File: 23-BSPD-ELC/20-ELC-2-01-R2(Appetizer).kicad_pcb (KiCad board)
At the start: 2 copper layers, 152.4 x 60.8 mm, 221 parts, among them J1 Conn_02x08_Counter_Clockwise, J2 Conn_01x02, J3 Conn_01x02, J4 SWD, Q1 Q_PMOS_GSD, Q2 Q_PMOS_GSD, Q3 Q_NMOS_GSD-Device, Q4 Q_NMOS_GSD-Device, Q5 Q_NMOS_GSD-Device, Q6 Q_NMOS_GSD-Device, Q7 Q_PMOS_DSG, Q8 Q_PMOS_DSG, SW1 SW_SPDT, U1 SN74ALS32DR, U10 LM239, U11 LM239, U13 LM239, U15 LM239, U16 STM32F105RCTx, U17 SN65HVD230, U18 SN65HVD230, U19 LMR51420, U2 74HC04D,653, U20 AMS1117-3.3, U3 74HC08D,653, U4 74LVC2G17DBVE4, U5 APX823-44W5G-7, U6 CD4043BDR, U8 LM239, Y1 16MHz

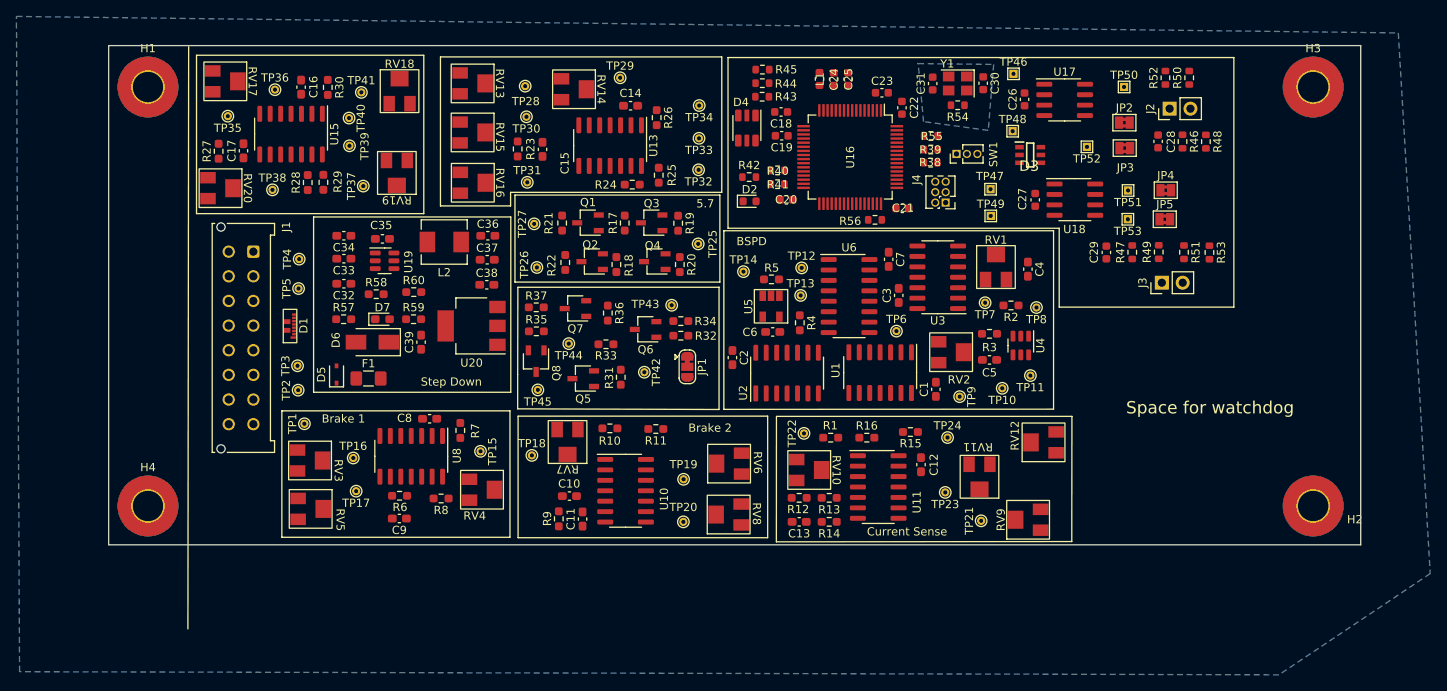
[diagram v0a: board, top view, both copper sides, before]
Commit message: BSPD layout
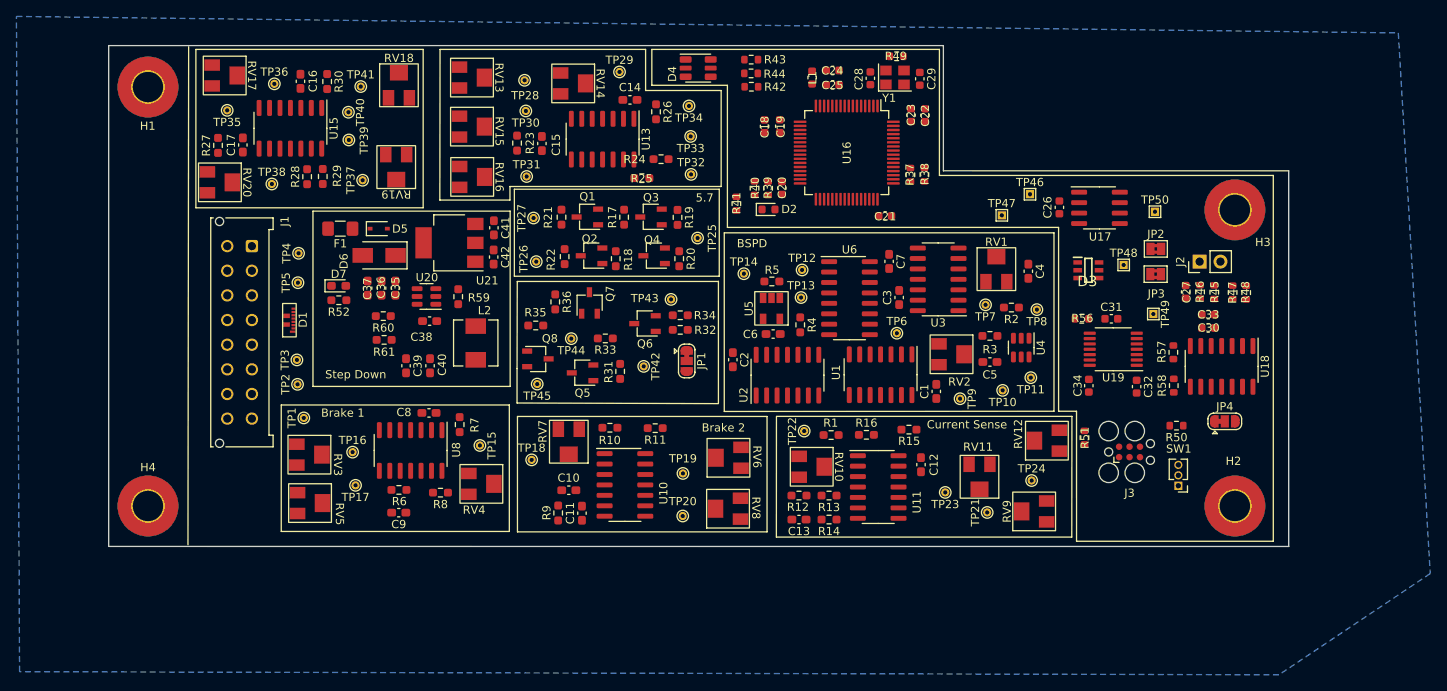
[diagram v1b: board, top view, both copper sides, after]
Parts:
- removed J4: SWD, Connector_PinHeader_1.27mm:PinHeader_2x03_P1.27mm_Vertical
- removed JP5: , Jumper:SolderJumper-2_P1.3mm_Bridged2Bar_Pad1.0x1.5mm
- removed R53: 120, Resistor_SMD:R_0603_1608Metric
- removed R54: 47, Resistor_SMD:R_0603_1608Metric
- removed R55: 10K, Resistor_SMD:R_0603_1608Metric
- removed TP51, TP52, TP53: , TestPoint:TestPoint_THTPad_1.0x1.0mm_Drill0.5mm
- added C40: 22uF, Capacitor_SMD:C_0603_1608Metric_Pad1.08x0.95mm_HandSolder, F.Cu at (106.3, 101.1)
- added C41: 1uF, Capacitor_SMD:C_0603_1608Metric_Pad1.08x0.95mm_HandSolder, F.Cu at (114.1, 84.3)
- added C42: 22uF, Capacitor_SMD:C_0603_1608Metric_Pad1.08x0.95mm_HandSolder, F.Cu at (114.1, 87.8)
- added R61: 54.9K, Resistor_SMD:R_0603_1608Metric_Pad0.98x0.95mm_HandSolder, F.Cu at (100.8, 97.9)
- added U21: AMS1117-3.3, Package_TO_SOT_SMD:SOT-223-3_TabPin2, F.Cu at (108.7, 86.1)
- C27: value 0u1 -> 4.7n
- C28, C29: value 4.7n -> 10p
- C30: value 10p -> .1uF
- C31: value 10p -> 1uF
- C32: value 10uF -> .1uF; footprint Capacitor_SMD:C_0603_1608Metric_Pad1.08x0.95mm_HandSolder -> Capacitor_SMD:C_0603_1608Metric
- C33: footprint Capacitor_SMD:C_0603_1608Metric_Pad1.08x0.95mm_HandSolder -> Capacitor_SMD:C_0603_1608Metric
- C34: value 100nF -> .1uF; footprint Capacitor_SMD:C_0603_1608Metric_Pad1.08x0.95mm_HandSolder -> Capacitor_SMD:C_0603_1608Metric
- C35: value 100nF -> 10uF
- C36: value 22uF -> 10uF
- C37: value 22uF -> 100nF
- C38: value 1uF -> 100nF
- J3: value Conn_01x02 -> SWD; footprint Connector_PinHeader_2.54mm:PinHeader_1x02_P2.54mm_Vertical -> Connector:Tag-Connect_TC2030-IDC-FP_2x03_P1.27mm_Vertical
- JP4: value (none) -> Jumper_3_Bridged12; footprint Jumper:SolderJumper-2_P1.3mm_Bridged2Bar_Pad1.0x1.5mm -> Jumper:SolderJumper-3_P1.3mm_Bridged12_RoundedPad1.0x1.5mm
- R19: value 250 -> 10k
- R37: value 25 -> 2k2; footprint Resistor_SMD:R_0603_1608Metric_Pad0.98x0.95mm_HandSolder -> Resistor_SMD:R_0603_1608Metric
- R41: value 2k2 -> 100
- R42: value 100 -> 220
- R45: value 220 -> 120
- R49: value 120 -> 47
- R50: value 120 -> 10K
- R51: value 120 -> 22
- R52: value 120 -> 470R; footprint Resistor_SMD:R_0603_1608Metric -> Resistor_SMD:R_0603_1608Metric_Pad0.98x0.95mm_HandSolder
- R56: value 22 -> 100k
- R57: value 470R -> 10k; footprint Resistor_SMD:R_0603_1608Metric_Pad0.98x0.95mm_HandSolder -> Resistor_SMD:R_0603_1608Metric
- R58: value 10K -> 10k; footprint Resistor_SMD:R_0603_1608Metric_Pad0.98x0.95mm_HandSolder -> Resistor_SMD:R_0603_1608Metric
- R60: value 54.9K -> 10K
- U18: value SN65HVD230 -> MCP3428; footprint Package_SO:SOIC-8_3.9x4.9mm_P1.27mm -> Package_SO:SOIC-14_3.9x8.7mm_P1.27mm
- U19: value LMR51420 -> LSF0204QPWRQ1; footprint Package_TO_SOT_SMD:SOT-23-6 -> Package_SO:TSSOP-14_4.4x5mm_P0.65mm
- U20: value AMS1117-3.3 -> LMR51420; footprint Package_TO_SOT_SMD:SOT-223-3_TabPin2 -> Package_TO_SOT_SMD:SOT-23-6
- moved C33 105.4 mm to (201.1, 94.8), turned to 0 degrees
- moved R52 104.2 mm to (95.2, 93.1), turned to 180 degrees
- moved R57 101.1 mm to (196.8, 99.4), turned to -90 degrees
- moved R58 97.7 mm to (196.9, 103.5), turned to 90 degrees
- moved C32 97.3 mm to (192.4, 103.6), turned to -90 degrees
- moved C34 92.5 mm to (186.5, 103.5), turned to -90 degrees
- moved U19 89.3 mm to (189.5, 99.1), turned to 180 degrees
- moved R45 61.3 mm to (201.8, 92.1), turned to -90 degrees
- moved SW1 48.6 mm to (197.4, 115.7), turned to 180 degrees
- moved R37 48.3 mm to (164.8, 77.8), turned to 90 degrees
- moved R50 42.4 mm to (197.2, 108.4), turned to 180 degrees
- moved C30 40.5 mm to (201.1, 96.5), turned to 0 degrees
- moved R49 39.8 mm to (163.1, 63.4), turned to 0 degrees
- moved C31 36.0 mm to (189.3, 95.4), turned to 0 degrees
- moved C28 35.9 mm to (159.9, 66.1)
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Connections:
- net /5.7/microcontroller/CAN1_H renamed /5.7/CANH
- net /5.7/microcontroller/CAN1_L renamed /5.7/CANL
- C27 pad 1: +3V3 -> GND
- C27 pad 2: GND -> Net-(C27-Pad2)
- C28 pad 1: GND -> /5.7/microcontroller/HSE_in
- C28 pad 2: Net-(C28-Pad2) -> GND
- C29 pad 1: GND -> Net-(C29-Pad1)
- C29 pad 2: Net-(C29-Pad2) -> GND
- C30 pad 1: /5.7/microcontroller/HSE_in -> +5V
- C32 pad 1: /24 to 5V Step Down/BUCK/V_in -> +3V3
- C33 pad 1: /24 to 5V Step Down/BUCK/V_in -> +5V
- C34 pad 1: /24 to 5V Step Down/BUCK/V_in -> +5V
- C35 pad 1: /24 to 5V Step Down/BUCK/SW -> /24 to 5V Step Down/BUCK/V_in
- C35 pad 2: /24 to 5V Step Down/BUCK/VBST -> GND
- C36 pad 1: +5V -> /24 to 5V Step Down/BUCK/V_in
- C37 pad 1: +5V -> /24 to 5V Step Down/BUCK/V_in
- C38 pad 1: +5V -> /24 to 5V Step Down/BUCK/SW
- C38 pad 2: GND -> /24 to 5V Step Down/BUCK/VBST
- C39 pad 1: +3V3 -> +5V
- D3 pad 1: Net-(D3-Pad1) -> unconnected-(D3-Pad1)
- D3 pad 3: Net-(D3-Pad3) -> unconnected-(D3-Pad3)
- J2 pad 1: Net-(C28-Pad2) -> Net-(C27-Pad2)
- J3 pad 1: Net-(C29-Pad2) -> +3V3
- JP4 pad 1: Net-(D3-Pad3) -> unconnected-(JP4-Pad1)
- JP4 pad 2: /5.7/microcontroller/CAN2_H -> Net-(JP4-Pad2)
- Q1 pad 3: /APPs1_Out -> /5.7/APPs1_Out
- Q2 pad 3: /APPs2_Out -> /5.7/APPs2_Out
- Q7 pad 2: /Shutdown_IN -> Net-(Q7-Pad2)
- Q7 pad 3: Net-(Q7-Pad3) -> /Shutdown_IN
- Q8 pad 2: Net-(Q8-Pad2) -> /Shutdown_OUT
- Q8 pad 3: /Shutdown_OUT -> Net-(Q7-Pad2)
- R21 pad 2: /APPs1_Out -> /5.7/APPs1_Out
- R22 pad 2: /APPs2_Out -> /5.7/APPs2_Out
- R35 pad 1: Net-(Q8-Pad2) -> Net-(Q7-Pad2)
- R37 pad 1: Net-(Q7-Pad3) -> +3V3
- R37 pad 2: Net-(Q8-Pad2) -> /5.7/microcontroller/I2C1_SCL
- R38 pad 2: /5.7/microcontroller/I2C1_SCL -> /5.7/microcontroller/I2C1_SDA
- R39 pad 2: /5.7/microcontroller/I2C1_SDA -> /5.7/microcontroller/I2C2_SCL
- R40 pad 2: /5.7/microcontroller/I2C2_SCL -> /5.7/microcontroller/I2C2_SDA
- R41 pad 1: +3V3 -> Net-(D2-Pad1)
- R41 pad 2: /5.7/microcontroller/I2C2_SDA -> GND
- R42 pad 1: Net-(D2-Pad1) -> Net-(D4-Pad6)
- R42 pad 2: GND -> /5.7/microcontroller/LED_B
- R43 pad 1: Net-(D4-Pad6) -> Net-(D4-Pad5)
- R43 pad 2: /5.7/microcontroller/LED_B -> /5.7/microcontroller/LED_G
- R44 pad 1: Net-(D4-Pad5) -> Net-(D4-Pad4)
- R44 pad 2: /5.7/microcontroller/LED_G -> /5.7/microcontroller/LED_R
- R45 pad 1: Net-(D4-Pad4) -> Net-(C27-Pad2)
- R45 pad 2: /5.7/microcontroller/LED_R -> Net-(D3-Pad4)
- R46 pad 1: Net-(C28-Pad2) -> Net-(C27-Pad2)
- R47 pad 1: Net-(C29-Pad2) -> Net-(D3-Pad6)
- R47 pad 2: Net-(D3-Pad1) -> Net-(J2-Pad2)
- R48 pad 1: Net-(C28-Pad2) -> Net-(D3-Pad6)
- R48 pad 2: Net-(D3-Pad4) -> Net-(J2-Pad2)
- R49 pad 1: Net-(C29-Pad2) -> /5.7/microcontroller/HSE_out
- R49 pad 2: Net-(D3-Pad1) -> Net-(C29-Pad1)
- R50 pad 1: Net-(D3-Pad6) -> Net-(R50-Pad1)
- R50 pad 2: Net-(J2-Pad2) -> /5.7/microcontroller/BOOT0
- R51 pad 1: Net-(D3-Pad3) -> Net-(J3-Pad2)
- R51 pad 2: Net-(J3-Pad2) -> /5.7/microcontroller/SWDIO
- R52 pad 1: Net-(D3-Pad6) -> GND
- R52 pad 2: Net-(J2-Pad2) -> Net-(D7-Pad1)
- R56 pad 1: Net-(J4-Pad2) -> Net-(C31-Pad1)
- R56 pad 2: /5.7/microcontroller/SWDIO -> +3V3
- R57 pad 1: GND -> /Watchdog/SDA
- R57 pad 2: Net-(D7-Pad1) -> +5V
- R58 pad 1: /24 to 5V Step Down/BUCK/V_in -> /Watchdog/SCL
- R58 pad 2: /24 to 5V Step Down/BUCK/EN -> +5V
- R59 pad 1: /24 to 5V Step Down/BUCK/VFB -> /24 to 5V Step Down/BUCK/V_in
- R59 pad 2: GND -> /24 to 5V Step Down/BUCK/EN
- R60 pad 2: +5V -> GND
- SW1 pad 2: Net-(R55-Pad1) -> Net-(R50-Pad1)
- TP1 pad 1: /Brake1_Signal_Raw -> /Brake2_Signal_Raw
- TP2 pad 1: /Current_Sense_Signal_Raw -> /Brake1_Signal_Raw
- TP26 pad 1: /APPs2_Out -> /5.7/APPs2_Out
- TP27 pad 1: /APPs1_Out -> /5.7/APPs1_Out
- TP3 pad 1: /Brake2_Signal_Raw -> /Current_Sense_Signal_Raw
- TP44 pad 1: Net-(Q7-Pad3) -> Net-(Q7-Pad2)
- TP47 pad 1: /5.7/microcontroller/CAN2_TX -> /5.7/microcontroller/CAN1_RX
- TP48 pad 1: /5.7/microcontroller/CAN1_RX -> Net-(D3-Pad6)
- TP49 pad 1: /5.7/microcontroller/CAN2_RX -> Net-(D3-Pad4)
- U16 pad 33: /5.7/microcontroller/CAN2_RX -> unconnected-(U16-Pad33)
- U16 pad 34: /5.7/microcontroller/CAN2_TX -> unconnected-(U16-Pad34)
- U18 pad 1: /5.7/microcontroller/CAN2_TX -> /Watchdog/CH1+
- U18 pad 3: +3V3 -> /Watchdog/CH2+
- U18 pad 4: /5.7/microcontroller/CAN2_RX -> GND
- U18 pad 5: unconnected-(U18-Pad5) -> GND
- U18 pad 6: Net-(D3-Pad1) -> +5V
- U18 pad 7: Net-(D3-Pad3) -> /Watchdog/SDA
- U18 pad 8: GND -> /Watchdog/SCL
- U19 pad 1: GND -> +3V3
- U19 pad 2: /24 to 5V Step Down/BUCK/SW -> /Watchdog/A1
- U19 pad 3: /24 to 5V Step Down/BUCK/V_in -> Net-(JP4-Pad2)
- U19 pad 4: /24 to 5V Step Down/BUCK/VFB -> /Watchdog/A3
- U19 pad 5: /24 to 5V Step Down/BUCK/EN -> /Watchdog/A4
- U19 pad 6: /24 to 5V Step Down/BUCK/VBST -> (no net)
- U20 pad 2: +3V3 -> /24 to 5V Step Down/BUCK/SW
- U20 pad 3: +5V -> /24 to 5V Step Down/BUCK/V_in
- Y1 pad 3: Net-(C31-Pad1) -> Net-(C29-Pad1)
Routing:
- removed copper zone on B.Cu, net (none)
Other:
- board size 152.4 x 60.8 mm -> 143.6 x 61 mm
- board text removed: "Space for watchdog"
